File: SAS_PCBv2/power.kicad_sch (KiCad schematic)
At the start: 17 parts, among them J3 Conn_01x02_Pin, Q2 AO3401A, Q3 AO3401A, SW1 SW_SPST, U2 SPX3819M5-L-3-3

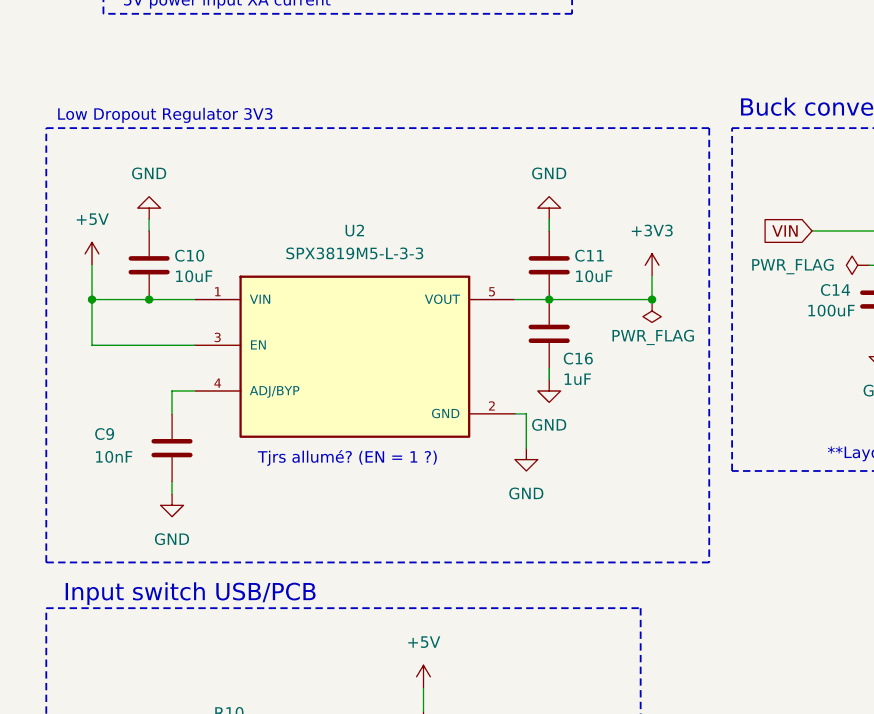
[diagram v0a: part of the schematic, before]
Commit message: LDO du service, Logic level shifter custom
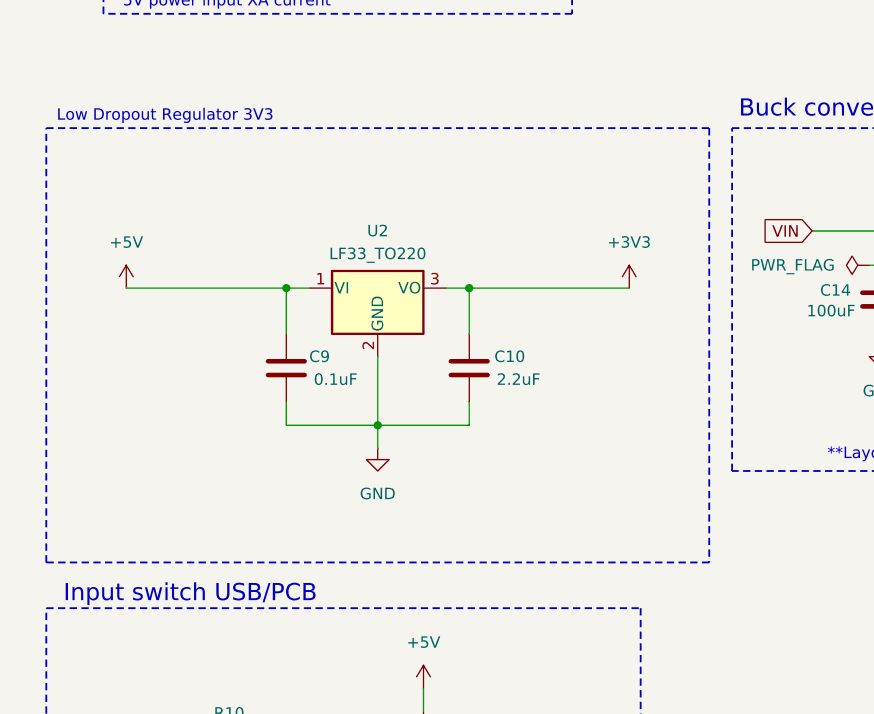
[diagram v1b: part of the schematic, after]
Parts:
- removed C11: 10uF, Capacitor_THT:CP_Radial_D5.0mm_P2.50mm, symbol Device:C
- removed C16: 1uF, Capacitor_THT:CP_Radial_D5.0mm_P2.50mm, symbol Device:C
- removed U2: SPX3819M5-L-3-3, Package_TO_SOT_SMD:SOT-23-5, symbol SAS_PCBv2_symbol:SPX3819M5-L-3-3
- added U2: LF33_TO220, Package_TO_SOT_THT:TO-220-3_Vertical, symbol Regulator_Linear:LF33_TO220
- C10: value 10uF -> 2.2uF; footprint Capacitor_THT:CP_Radial_D5.0mm_P2.50mm -> SAS_PCBv2_footprint:CAP_FG14_TDK
- C9: value 10nF -> 0.1uF; footprint Capacitor_THT:C_Disc_D5.0mm_W2.5mm_P2.50mm -> SAS_PCBv2_footprint:CAP_C320_KEM
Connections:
- net +3V3: now also C10.1, U2.3 (VO)
- net +5V: now also C9.1, U2.1 (VI); no longer C10.2
- net GND: now also C10.2, U2.2 (GND); no longer C10.1
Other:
- note removed: "Tjrs allumé? (EN = 1 ?)"
